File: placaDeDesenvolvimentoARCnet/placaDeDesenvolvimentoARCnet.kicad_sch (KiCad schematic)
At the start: 6 parts, among them J1 Txs0108e I2c, J2 Conn_01x23_Socket, J4 BeagleBoneBlakc, P1 Conn_01x23_Socket, P2 Conn_01x23_Socket, U2 COM20020I-DZD

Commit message: 07deJan atualizacao
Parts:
- added C1, C2, C3, C4: 33pf, symbol Device:C
- added J2: Txs0108e control, symbol Connector_Generic_MountingPin:Conn_02x10_Counter_Clockwise_MountingPin
- added J3: Txs0108e network, symbol Connector_Generic_MountingPin:Conn_02x10_Counter_Clockwise_MountingPin
- added JP1, JP2, JP3, JP4: ~, symbol Jumper:Jumper_2_Open
- added R1: 1k, symbol Device:R
- added R2, R3, R4: 10K, symbol Device:R_Small_US
- added U1: TXS0108EPWR, TXS0108EPWR:SOP65P640X120-20N, symbol TXS0108EPWR:TXS0108EPWR
- added U3: BBB01-SC-505, MODULE_BBB01-SC-505, symbol BBB01-SC-5016:BBB01-SC-505
- added Y1: 20Mhz, symbol Device:Crystal
- added Y2: 40Mhz, symbol Device:Crystal
- J1: value Txs0108e I2c -> Txs0108e I/O
- renumbered P2 to P8, P1 to P9
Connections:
- net D5B3: now reaches U2.10 (D5)
- net D5B3: now also J1.B3 (BPin_7)
- net D6B2: now reaches U2.11 (D6)
- net D6B2: now also J1.B2 (Pin_8)
- net D7B1: now reaches U2.12 (D7)
- net D7B1: now also J1.B1 (Pin_9)
- net +5V: now reaches U2.15 (VDD)
- net +5V: now also J1.VB (Pin_10), J2.VB (Pin_10), J3.VB (Pin_10)
- net at U2.16 (XTAL1): now also JP1.1 (A), JP3.1 (A)
- net at U2.17 (XTAL2): now also JP2.1 (A), JP4.1 (A)
- net at U2.18 (~{PULSE1}): now also J3.B1 (Pin_9)
- net at U2.19 (~{PULSE2}): now also J3.B2 (Pin_8)
- net at U2.20 (RXIN): now also J3.B4 (Pin_6)
- net at U2.21 (~{TXEN}): now also J3.B3 (BPin_7)
- net at U2.23 (~{RESET_IN}): now also J2.B7 (Pin_3)
- net at U2.24 (~{INTR}): now also J2.B2 (Pin_8)
- net at U2.25 (~{CS}): now also J2.B1 (Pin_9)
- net at U2.26 (~{WR}/DIR): now also J2.B6 (Pin_4)
- net at U2.27 (~{RD}/~{DS}): now also J2.BB (Pin_2)
- net AD0B8: now reaches U2.4 (AD0)
- net AD1B7: now reaches U2.5 (AD1)
- net AD2B6: now reaches U2.6 (AD2)
- net GND: now reaches U2.7 (VSS)
- net GND: now also J1.GND (Pin_1), C1.1, C2.1, C3.1, C4.1, J2.GND (Pin_1), J3.GND (Pin_1), U3.P9_1 (GND_P9_1)
- net D3B5: now reaches U2.8 (D3)
- net D4B4: now reaches U2.9 (D4)
- net P9_18: now reaches J1.A1 (APin_12)
- net P9_18: now also U3.P9_18 (I2C1_SDA)
- net P9_17: now reaches J1.A2 (Pin_13)
- net P9_17: now also U3.P9_17 (I2C1_SCL)
- net P9_16: now reaches J1.A3 (Pin_14)
- net P9_16: now also U3.P9_16 (EHRPWM1B)
- net P9_15: now reaches J1.A4 (Pin_15)
- net P9_15: now also U3.P9_15 (GPIO1_16)
- net P9_14: now reaches J1.A5 (Pin_16)
- net P9_14: now also U3.P9_14 (EHRPWM1A)
- net P9_13: now reaches J1.A6 (Pin_17)
- net P9_13: now also U3.P9_13 (UART4_TXD)
- net P9_12: now reaches J1.A7 (Pin_18)
- net P9_12: now also U3.P9_12 (GPIO1_28)
- net P9_11: now reaches J1.AB (Pin_19)
- net P9_11: now also U3.P9_11 (UART4_RXD)
- net D4_5V: now reaches J1.B4 (Pin_6)
- net D3_5V: now reaches J1.B5 (Pin_5)
- net AD2_5V: now reaches J1.B6 (Pin_4)
- net AD1_5V: now reaches J1.B7 (Pin_3)
- net AD0_5V: now reaches J1.BB (Pin_2)
- net at J1.DE (Pin_20): now also R2.1
- net at J1.VA (Pin_11): now also J2.VA (Pin_11), J3.VA (Pin_11), R2.2, R3.2, R4.2, U3.P9_3 (DC_3.3V_P9_3)
- net at P9.22 (Pin_22): now also U1.12 (B8)
- net at P9.23 (Pin_23): now also U1.11 (GND)
- new net: C1.2, JP2.2 (B), Y1.1
- new net: C2.2, JP1.2 (B), Y1.2
- new net: J2.DE (Pin_20), R3.1
- new net: J3.DE (Pin_20), R4.1
- new net: C4.2, R1.1, Y2.1
- new net: C3.2, R1.2, Y2.2
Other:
- sheet Untitled Sheet renamed 2
- note added: "+3V3"
- note added: "+5V"
- note added: "CS"
- note added: "INTR"
- note added: "PULSE1"
- note added: "PULSE2"
- note added: "RD/DS"
- note added: "RESET"
- note added: "RX"
- note added: "TX"
- note added: "WR/DIR"
- moved on the sheet: J1, P8, P9, U2

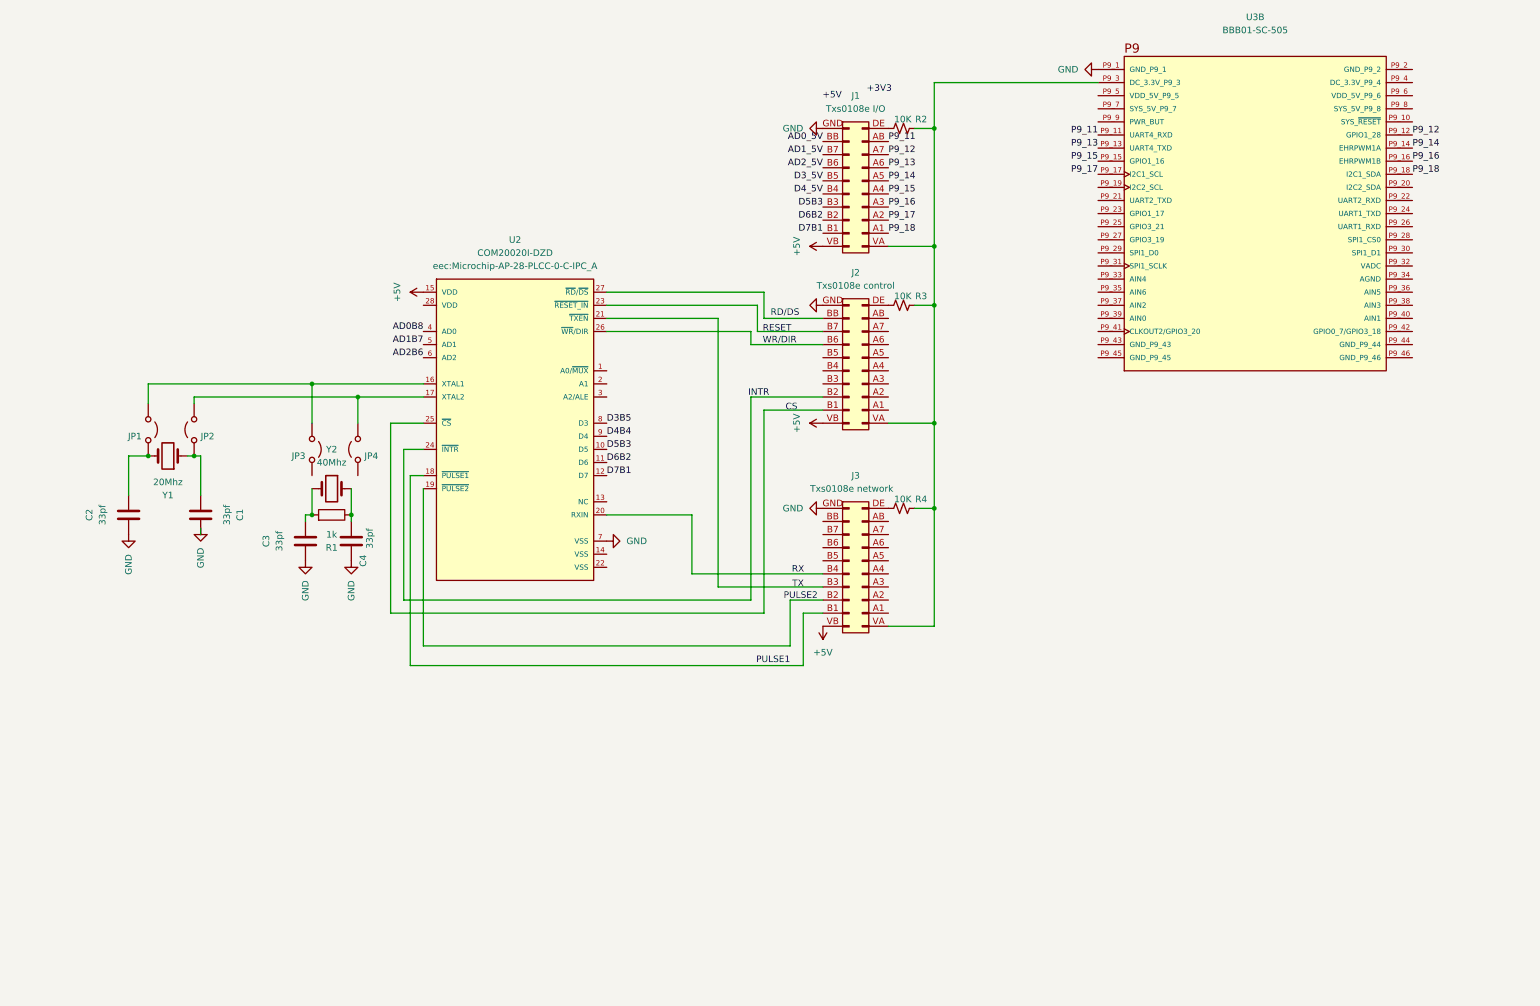
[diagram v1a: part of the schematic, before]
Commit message: atualização esquematico
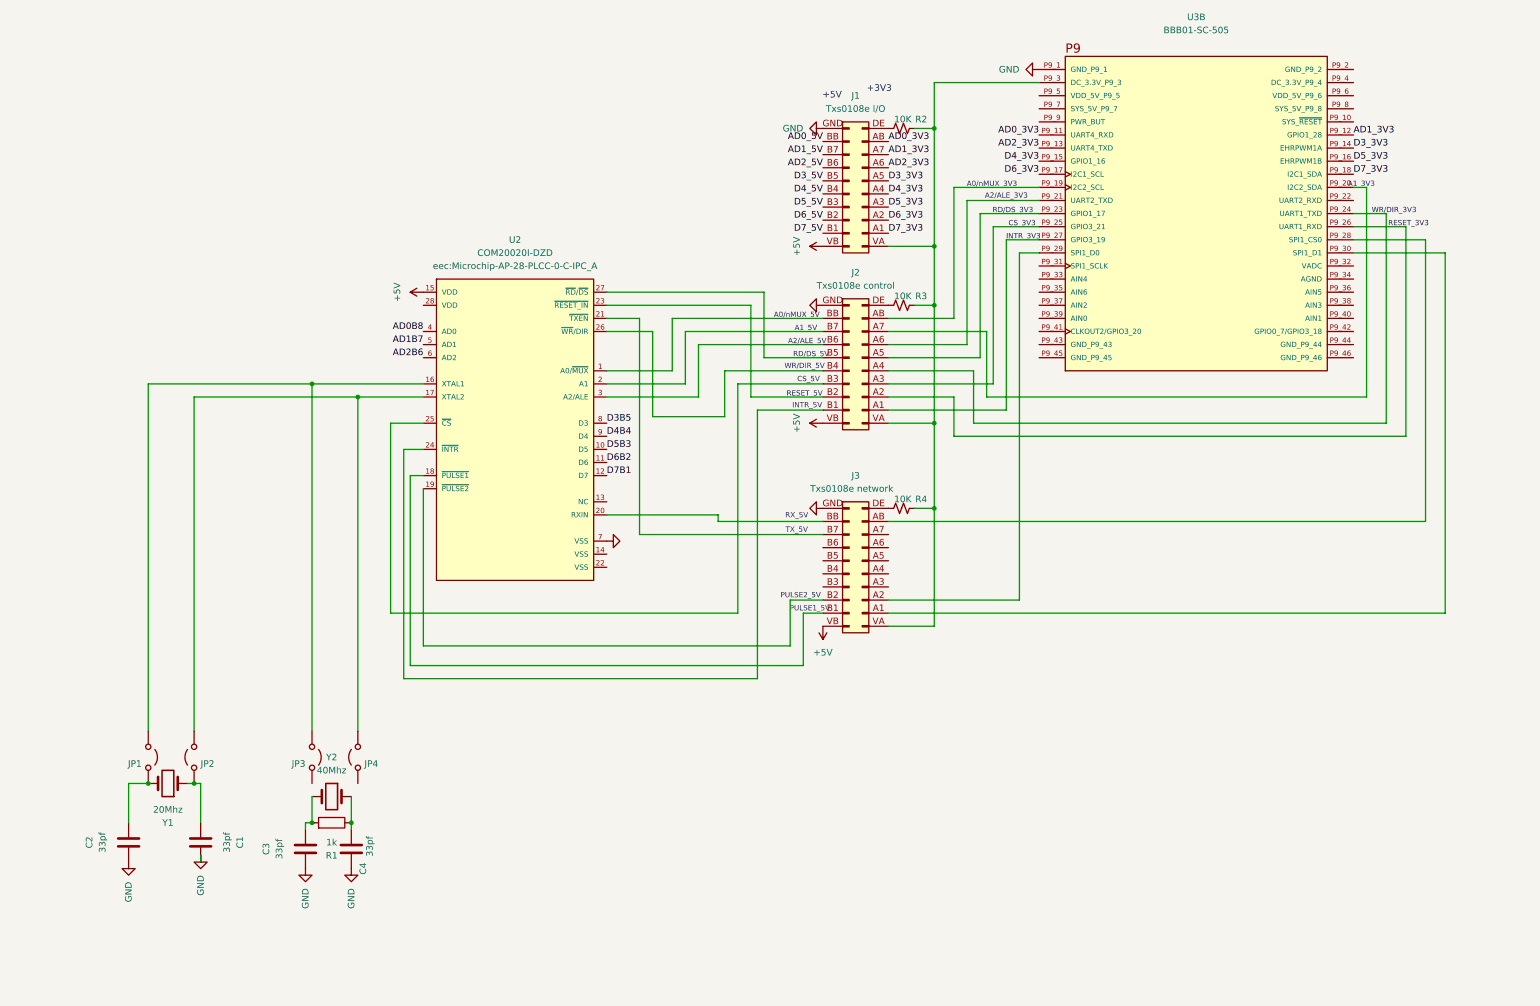
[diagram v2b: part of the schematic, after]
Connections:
- net D5B3: no longer J1.B3 (BPin_7)
- net D6B2: no longer J1.B2 (Pin_8)
- net D7B1: no longer J1.B1 (Pin_9)
- net at U3.P9_19 (I2C2_SCL): now also J2.AB (Pin_19)
- net at U3.P9_20 (I2C2_SDA): now also J2.A7 (Pin_18)
- net at U3.P9_21 (UART2_TXD): now also J2.A6 (Pin_17)
- net at U3.P9_23 (GPIO1_17): now also J2.A5 (Pin_16)
- net at U3.P9_24 (UART1_TXD): now also J2.A4 (Pin_15)
- net at U3.P9_25 (GPIO3_21): now also J2.A3 (Pin_14)
- net at U3.P9_26 (UART1_RXD): now also J2.A2 (Pin_13)
- net at U3.P9_27 (GPIO3_19): now also J2.A1 (APin_12)
- net at U3.P9_28 (SPI1_CS0): now also J3.AB (Pin_19)
- net at U3.P9_29 (SPI1_D0): now also J3.A2 (Pin_13)
- net at U3.P9_30 (SPI1_D1): now also J3.A1 (APin_12)
- net at J2.B1 (Pin_9): now also U2.24 (~{INTR}); no longer U2.25 (~{CS})
- net at J2.B2 (Pin_8): now also U2.23 (~{RESET_IN}); no longer U2.24 (~{INTR})
- net at J2.B3 (BPin_7): now also U2.25 (~{CS})
- net at J2.B4 (Pin_6): now also U2.26 (~{WR}/DIR)
- net at J2.B5 (Pin_5): now also U2.27 (~{RD}/~{DS})
- net at J2.B6 (Pin_4): now also U2.3 (A2/ALE); no longer U2.26 (~{WR}/DIR)
- net at J2.B7 (Pin_3): now also U2.2 (A1); no longer U2.23 (~{RESET_IN})
- net at J2.BB (Pin_2): now also U2.1 (A0/~{MUX}); no longer U2.27 (~{RD}/~{DS})
- net at J3.B3 (BPin_7): no longer U2.21 (~{TXEN})
- net at J3.B4 (Pin_6): no longer U2.20 (RXIN)
- net at J3.B7 (Pin_3): now also U2.21 (~{TXEN})
- net at J3.BB (Pin_2): now also U2.20 (RXIN)
- net P9_11 renamed AD0_3V3
- net P9_12 renamed AD1_3V3
- net P9_13 renamed AD2_3V3
- net P9_14 renamed D3_3V3
- net P9_15 renamed D4_3V3
- net P9_16 renamed D5_3V3
- net P9_17 renamed D6_3V3
- net P9_18 renamed D7_3V3
- new net D5_5V: J1.B3 (BPin_7)
- new net D6_5V: J1.B2 (Pin_8)
- new net D7_5V: J1.B1 (Pin_9)
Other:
- note added: "A0/nMUX_3V3"
- note added: "A0/nMUX_5V"
- note added: "A1_3V3"
- note added: "A1_5V"
- note added: "A2/ALE_3V3"
- note added: "A2/ALE_5V"
- note added: "CS_3V3"
- note added: "CS_5V"
- note added: "INTR_3V3"
- note added: "INTR_5V"
- note added: "PULSE1_5V"
- note added: "PULSE2_5V"
- note added: "RD/DS_3V3"
- note added: "RD/DS_5V"
- note added: "RESET_3V3"
- note added: "RESET_5V"
- note added: "RX_5V"
- note added: "TX_5V"
- note added: "WR/DIR_3V3"
- note added: "WR/DIR_5V"
- note removed: "CS"
- note removed: "INTR"
- note removed: "PULSE1"
- note removed: "PULSE2"
- note removed: "RD/DS"
- note removed: "RESET"
- note removed: "RX"
- note removed: "TX"
- note removed: "WR/DIR"
- moved on the sheet: C1, C2, C3, C4, JP1, JP2, JP3, JP4, R1, U3B, Y1, Y2
